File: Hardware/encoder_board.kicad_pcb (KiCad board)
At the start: 4 copper layers, 20.8 x 39.1 mm, 29 parts, among them J1 Conn_01x02_Female, J2 Conn_01x04_Male, J3 Conn_01x05_Male, J5 Conn_01x01_Female, J6 Conn_01x01_Female, SW1 SW_Push, U1 LP2985-3.3, U2 HCMS-2903, U3 STM32F410RBTx

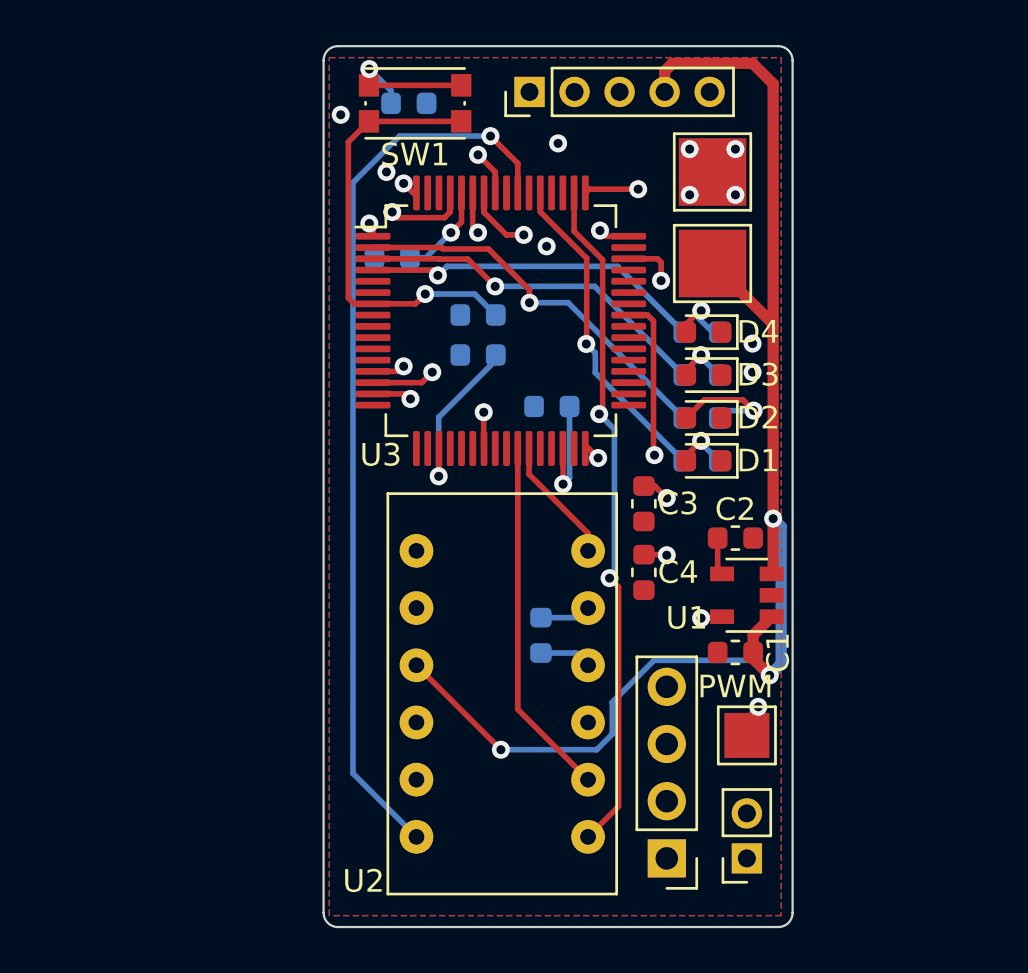
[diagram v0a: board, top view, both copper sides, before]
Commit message: Board ordered.
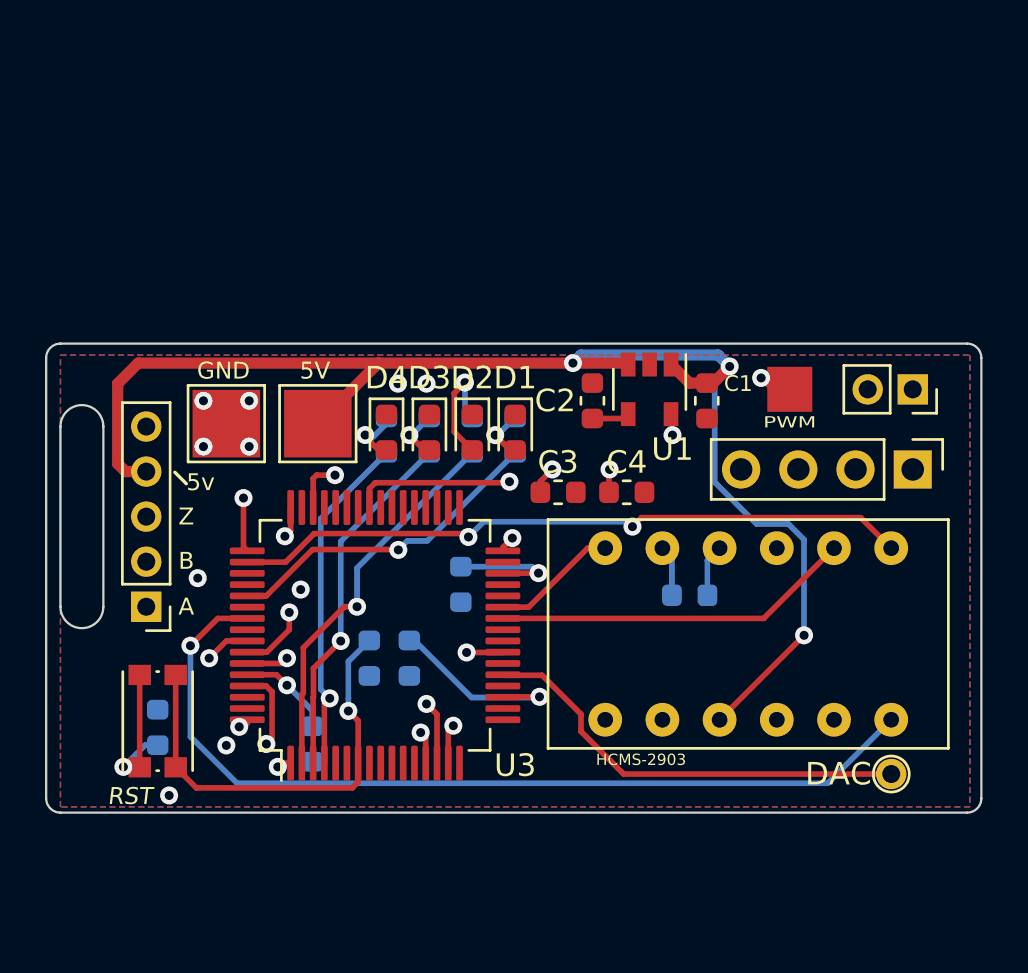
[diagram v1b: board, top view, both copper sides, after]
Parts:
- added DAC: Conn_01x01_Female, TestPoint:TestPoint_Plated_Hole_D2.0mm, F.Cu at (165.3, 109.0)
- moved R6 29.9 mm to (132.7, 107.0), turned to 270 degrees
- moved RST 29.7 mm to (132.7, 106.7), turned to 90 degrees
- moved J3 28.5 mm to (132.2, 101.6), turned to 180 degrees
- moved J5 24.3 mm to (135.8, 93.5), turned to 90 degrees
- moved J1 22.1 mm to (166.2, 91.9), turned to 270 degrees
- moved R7 21.9 mm to (139.6, 107.7), turned to 90 degrees
- moved J2 20.4 mm to (166.2, 95.5), turned to 270 degrees
- moved J6 18.9 mm to (139.8, 93.5), turned to 90 degrees
- moved G*** 17.5 mm to (130.0, 105.2)
- moved C6 16.0 mm to (142.1, 103.9), turned to 270 degrees
- moved PWM 15.5 mm to (160.8, 91.9), turned to 90 degrees
- moved U3 15.0 mm to (142.4, 102.9), turned to 90 degrees
- moved D4 14.8 mm to (142.9, 93.9), turned to 270 degrees
- moved R4 14.7 mm to (142.9, 94.0), turned to 90 degrees
- moved C5 13.8 mm to (143.9, 103.9), turned to 270 degrees
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- renumbered U2 to HCMS-2903, SW1 to RST
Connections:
- U3 pad 21: (no net) -> DAC_1
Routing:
- net DAC_1: track 0.00 -> 19.5 mm
- net +3V3: track 18.1 -> 18.7 mm
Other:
- board size 20.8 x 39.1 mm -> 41.5 x 20.8 mm
- rule via_min_size: 0.4 -> 0.254
- board text added: "5V"
- board text added: "5v"
- board text added: "A"
- board text added: "B"
- board text added: "GND"
- board text added: "Z"
